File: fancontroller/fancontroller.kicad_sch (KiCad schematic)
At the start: 9 parts, among them SW1 SW_RESET, SW2 SW_BOOT, U1 ESP32-WROOM-32, U2 AMS1117-3.3

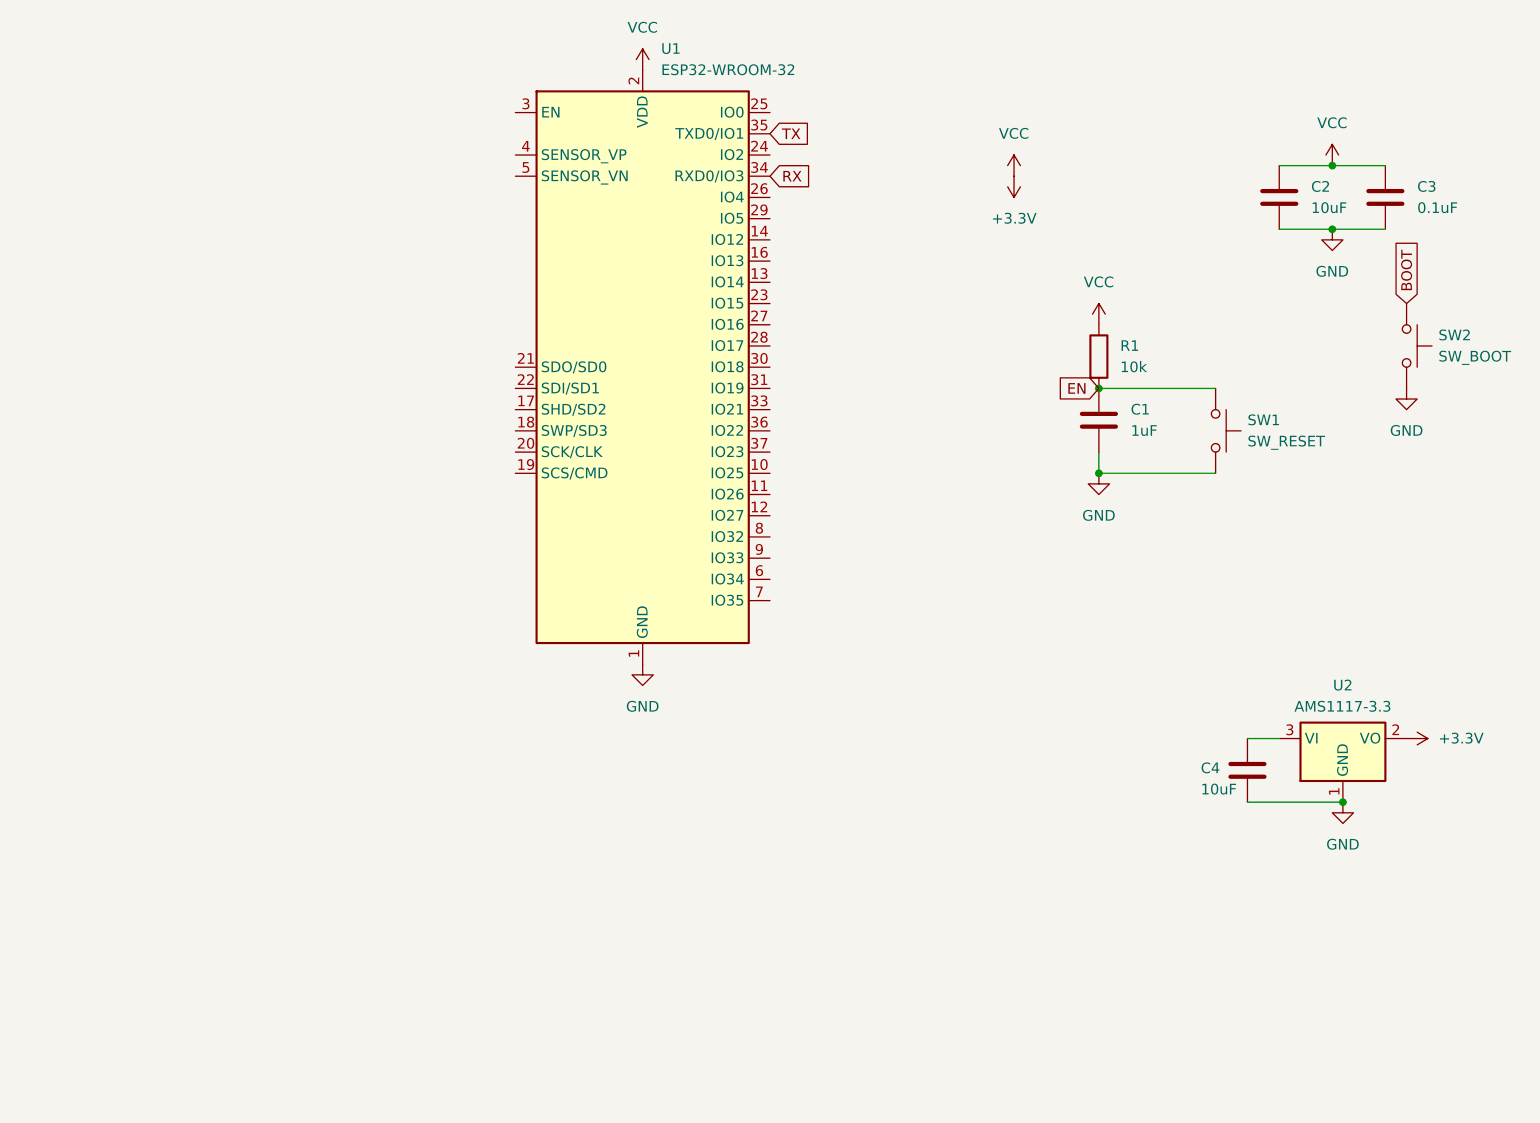
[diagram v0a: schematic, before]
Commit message: KIcad messing
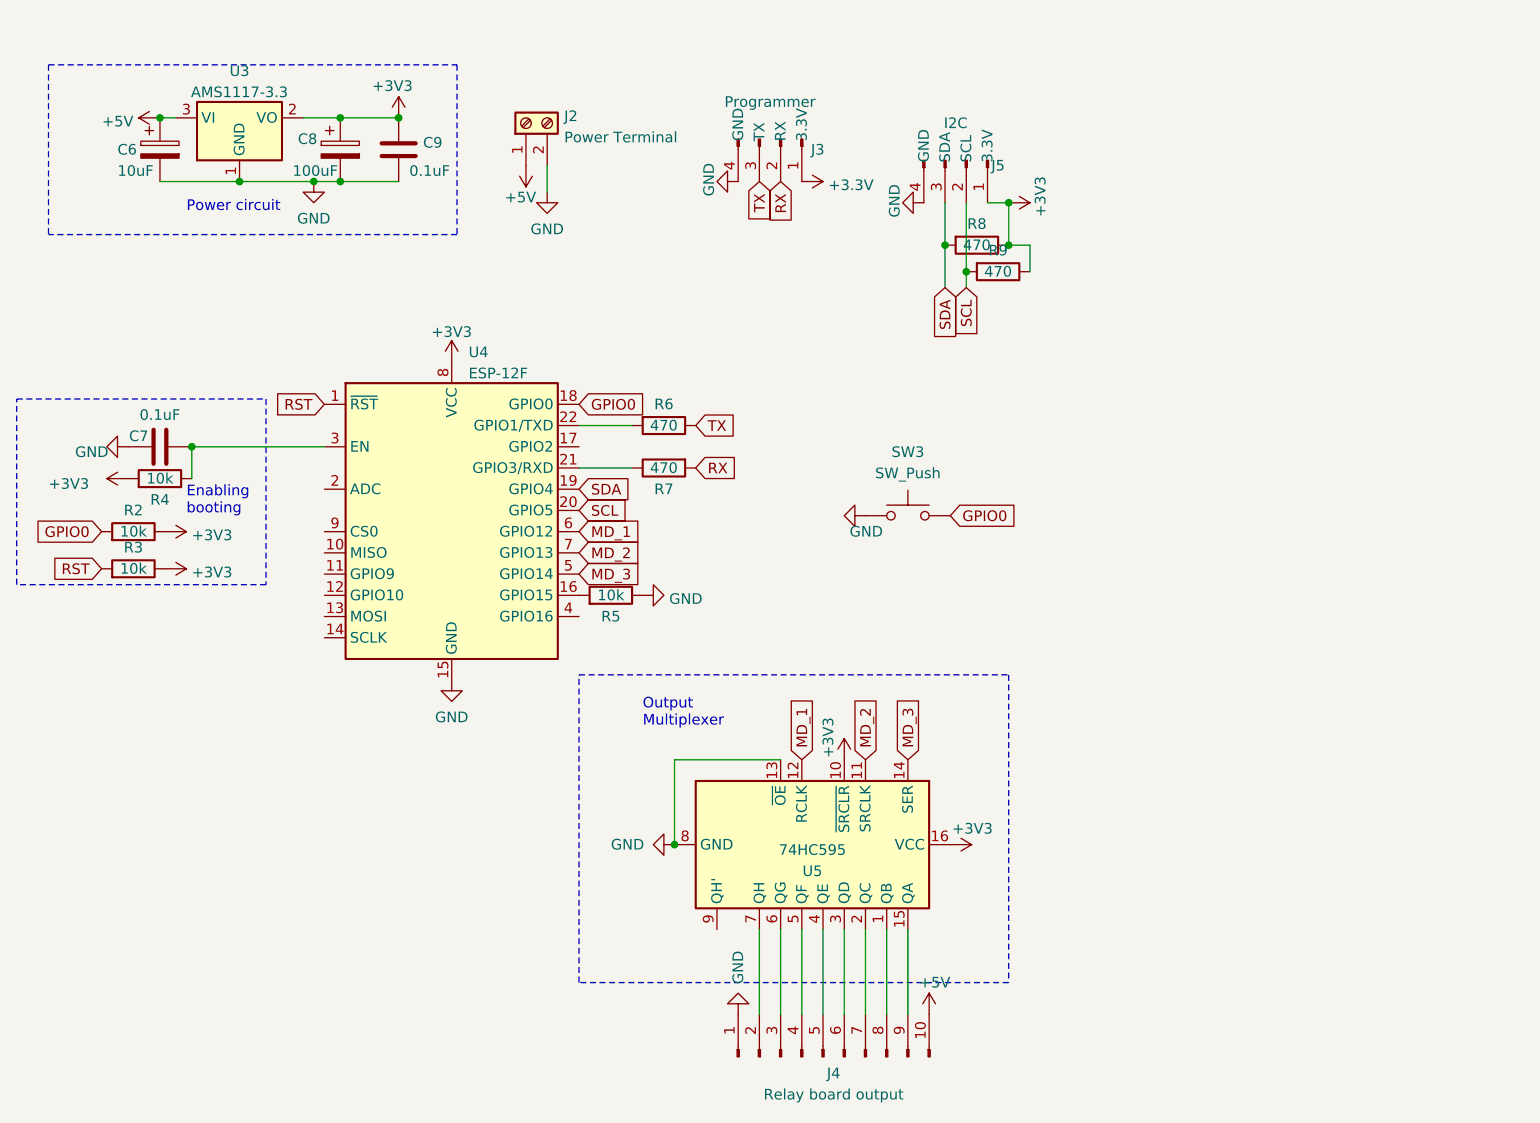
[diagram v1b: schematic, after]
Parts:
- removed C1: 1uF, symbol Device:C
- removed C2, C4: 10uF, symbol Device:C
- removed C3: 0.1uF, symbol Device:C
- removed R1: 10k, symbol Device:R
- removed SW1: SW_RESET, symbol Switch:SW_Push
- removed SW2: SW_BOOT, symbol Switch:SW_Push
- removed U1: ESP32-WROOM-32, RF_Module:ESP32-WROOM-32, symbol RF_Module:ESP32-WROOM-32
- removed U2: AMS1117-3.3, Package_TO_SOT_SMD:SOT-223-3_TabPin2, symbol Regulator_Linear:AMS1117-3.3
- added C6: 10uF, Capacitor_THT:CP_Radial_D4.0mm_P1.50mm, symbol Device:C_Polarized
- added C7, C9: 0.1uF, Capacitor_THT:C_Disc_D3.0mm_W2.0mm_P2.50mm, symbol Device:C
- added C8: 100uF, Capacitor_THT:CP_Radial_D5.0mm_P2.00mm, symbol Device:C_Polarized
- added J2: Power Terminal, TerminalBlock:TerminalBlock_bornier-2_P5.08mm, symbol Connector:Screw_Terminal_01x02
- added J3: Programmer, Connector_PinHeader_2.54mm:PinHeader_1x04_P2.54mm_Vertical, symbol Connector:Conn_01x04_Male
- added J4: Relay board output, Connector_PinHeader_2.54mm:PinHeader_1x10_P2.54mm_Vertical, symbol Connector:Conn_01x10_Male
- added J5: I2C, Connector_PinHeader_2.54mm:PinHeader_1x04_P2.54mm_Vertical, symbol Connector:Conn_01x04_Male
- added R2, R3, R4, R5: 10k, Resistor_THT:R_Axial_DIN0207_L6.3mm_D2.5mm_P7.62mm_Horizontal, symbol Device:R
- added R6, R7, R8, R9: 470, Resistor_THT:R_Axial_DIN0207_L6.3mm_D2.5mm_P7.62mm_Horizontal, symbol Device:R
- added SW3: SW_Push, symbol Switch:SW_Push
- added U3: AMS1117-3.3, Package_TO_SOT_SMD:SOT-223-3_TabPin2, symbol Regulator_Linear:AMS1117-3.3
- added U4: ESP-12F, RF_Module:ESP-12E, symbol RF_Module:ESP-12F
- added U5: 74HC595, Package_DIP:DIP-16_W7.62mm_Socket, symbol 74xx:74HC595
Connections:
- net +3.3V: now also J3.1 (Pin_1)
- net GND: now also C6.2, C7.1, C8.2, C9.2, J2.2 (Pin_2), J3.4 (Pin_4), J4.1 (Pin_1), J5.4 (Pin_4), R5.1, SW3.1, U3.1 (GND), U4.15 (GND), U5.13 (~{OE}), U5.8 (GND)
- net RX: now also J3.2 (Pin_2), R7.2
- net TX: now also J3.3 (Pin_3), R6.1
- new net: J4.8 (Pin_8), U5.1 (QB)
- new net: J4.9 (Pin_9), U5.15 (QA)
- new net: J4.7 (Pin_7), U5.2 (QC)
- new net: J4.6 (Pin_6), U5.3 (QD)
- new net: J4.5 (Pin_5), U5.4 (QE)
- new net: J4.4 (Pin_4), U5.5 (QF)
- new net: J4.3 (Pin_3), U5.6 (QG)
- new net: J4.2 (Pin_2), U5.7 (QH)
- new net: R5.2, U4.16 (GPIO15)
- new net: R7.1, U4.21 (GPIO3/RXD)
- new net: R6.2, U4.22 (GPIO1/TXD)
- new net: C7.2, R4.1, U4.3 (EN)
- new net +3V3: C8.1, C9.1, J5.1 (Pin_1), R2.1, R3.1, R4.2, R8.1, R9.1, U3.2 (VO), U4.8 (VCC), U5.10 (~{SRCLR}), U5.16 (VCC)
- new net +5V: C6.1, J2.1 (Pin_1), J4.10 (Pin_10), U3.3 (VI)
- new net GPIO0: R2.2, SW3.2, U4.18 (GPIO0)
- new net MD_1: U4.6 (GPIO12), U5.12 (RCLK)
- new net MD_2: U4.7 (GPIO13), U5.11 (SRCLK)
- new net MD_3: U4.5 (GPIO14), U5.14 (SER)
- new net RST: R3.2, U4.1 (~{RST})
- new net SCL: J5.2 (Pin_2), R9.2, U4.20 (GPIO5)
- new net SDA: J5.3 (Pin_3), R8.2, U4.19 (GPIO4)
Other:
- note added: "Enabling booting"
- note added: "Output Multiplexer"
- note added: "Power circuit"
